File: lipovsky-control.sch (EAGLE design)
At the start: 45 parts, among them J5 AVRISP0.1", P1 M04-929P, P2 M04-929P, P3 M04-929P, P4 M04-929P, U1 ATTINYX4A8MU, U2 MIC2288YD5, U3 MIC2288YD5, U4 LTV-816S

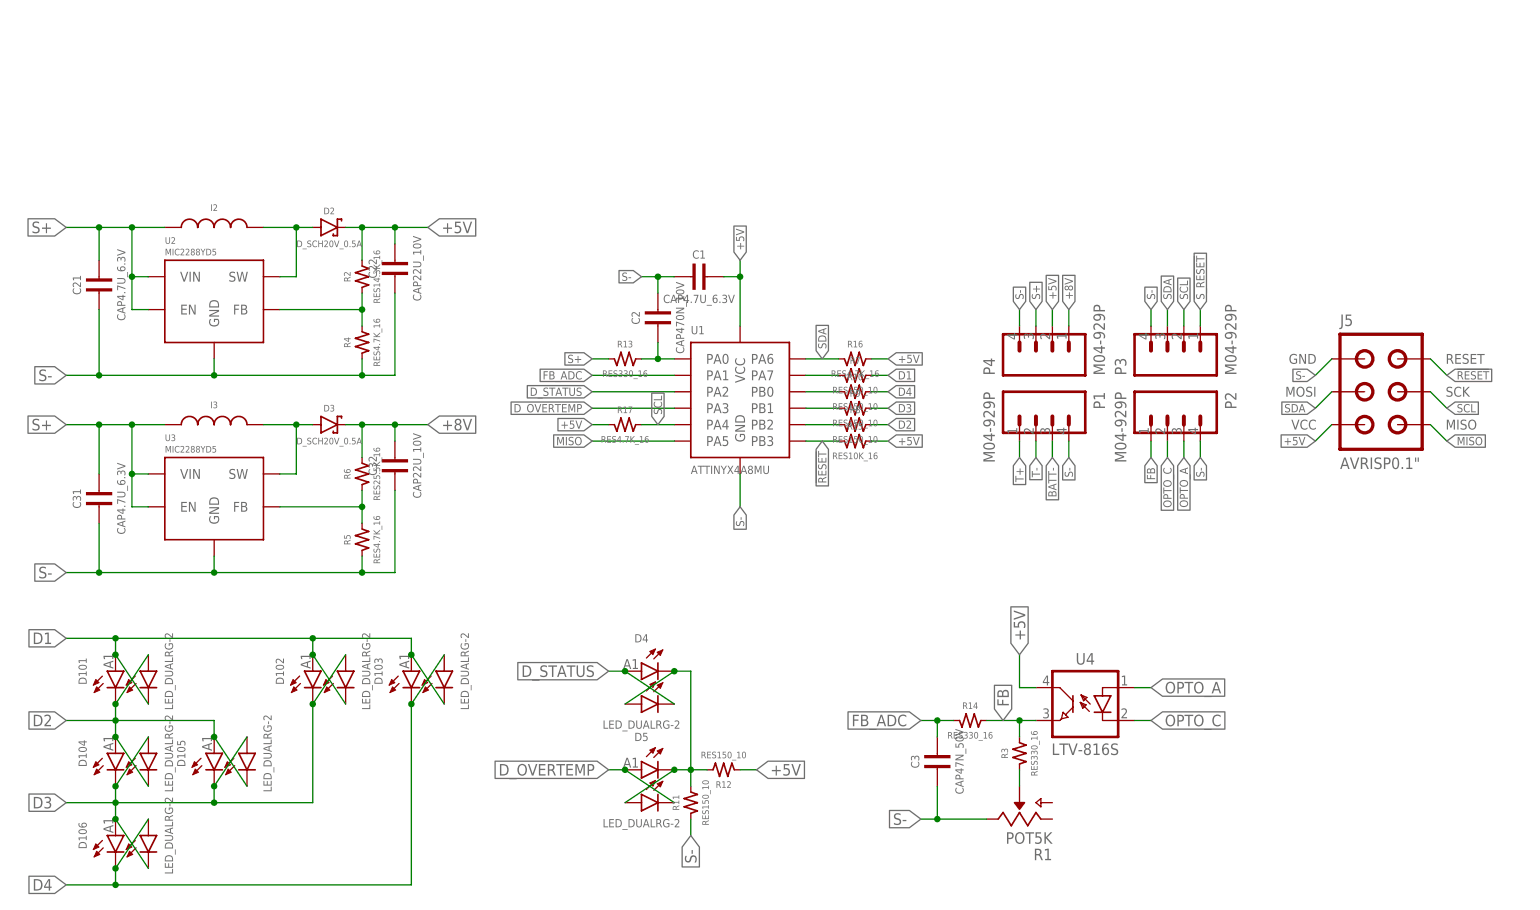
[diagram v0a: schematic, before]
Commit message: tweaks
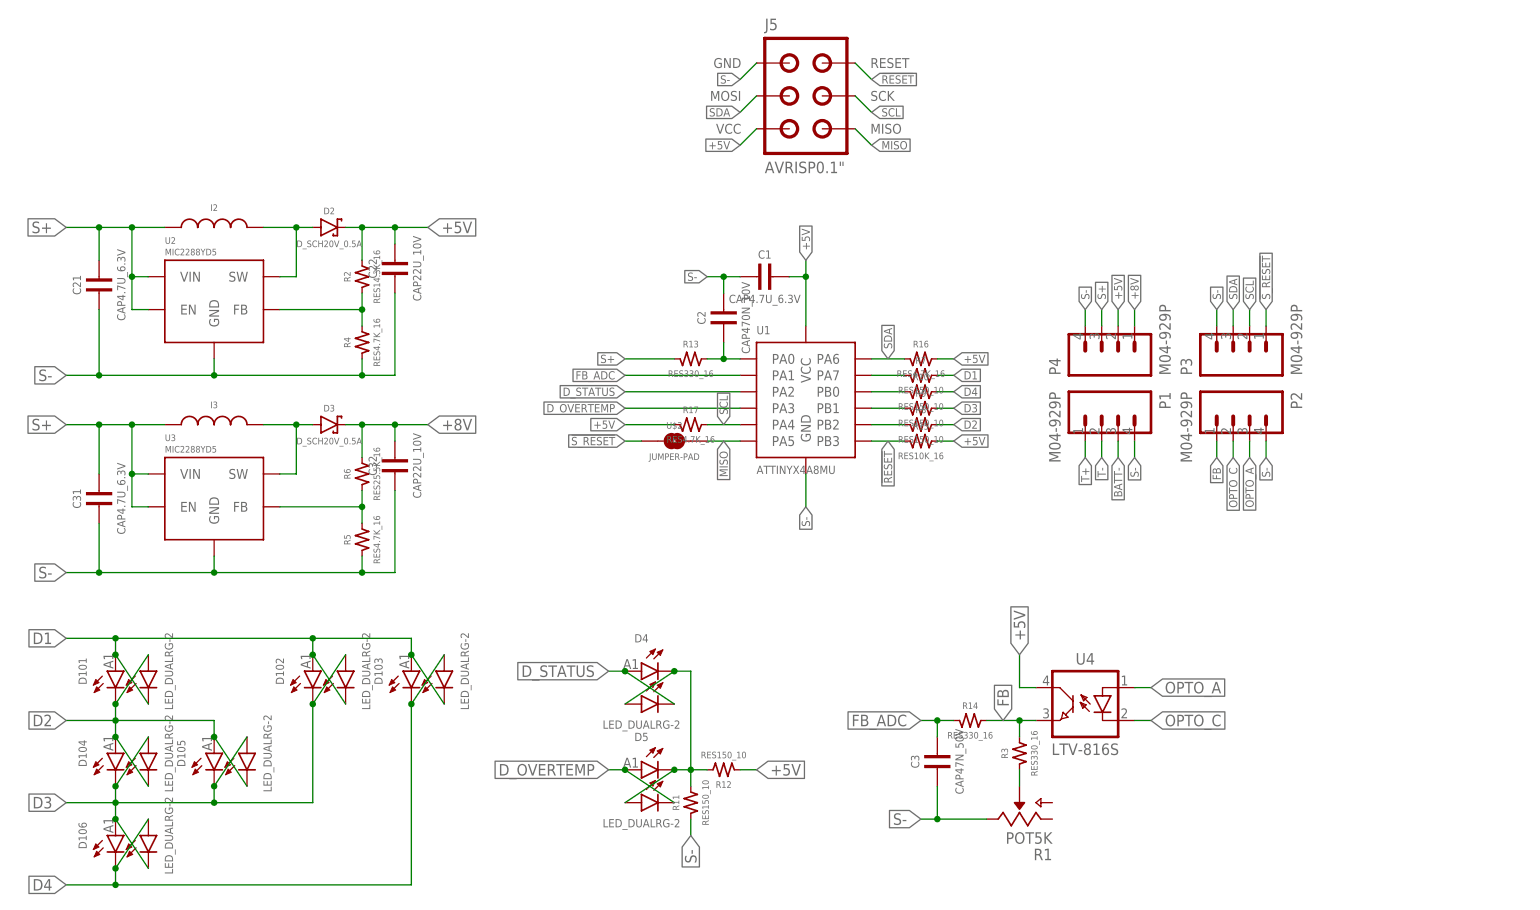
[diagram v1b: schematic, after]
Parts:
- added U$2: JUMPER-PAD, dubec:JUMPER-PAD
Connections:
- net !S_RESET: now also U$2.1
- net MISO: now also U$2.2
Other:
- moved on the sheet: C1, C2, J5, P1, P2, P3, P4, R10, R13, R15, R16, R17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
